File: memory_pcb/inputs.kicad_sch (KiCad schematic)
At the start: 12 parts, among them SW1 SW_Push, SW2 SW_Push, SW3 RotaryEncoder_Switch, U3 100SP3T2B4M6RE

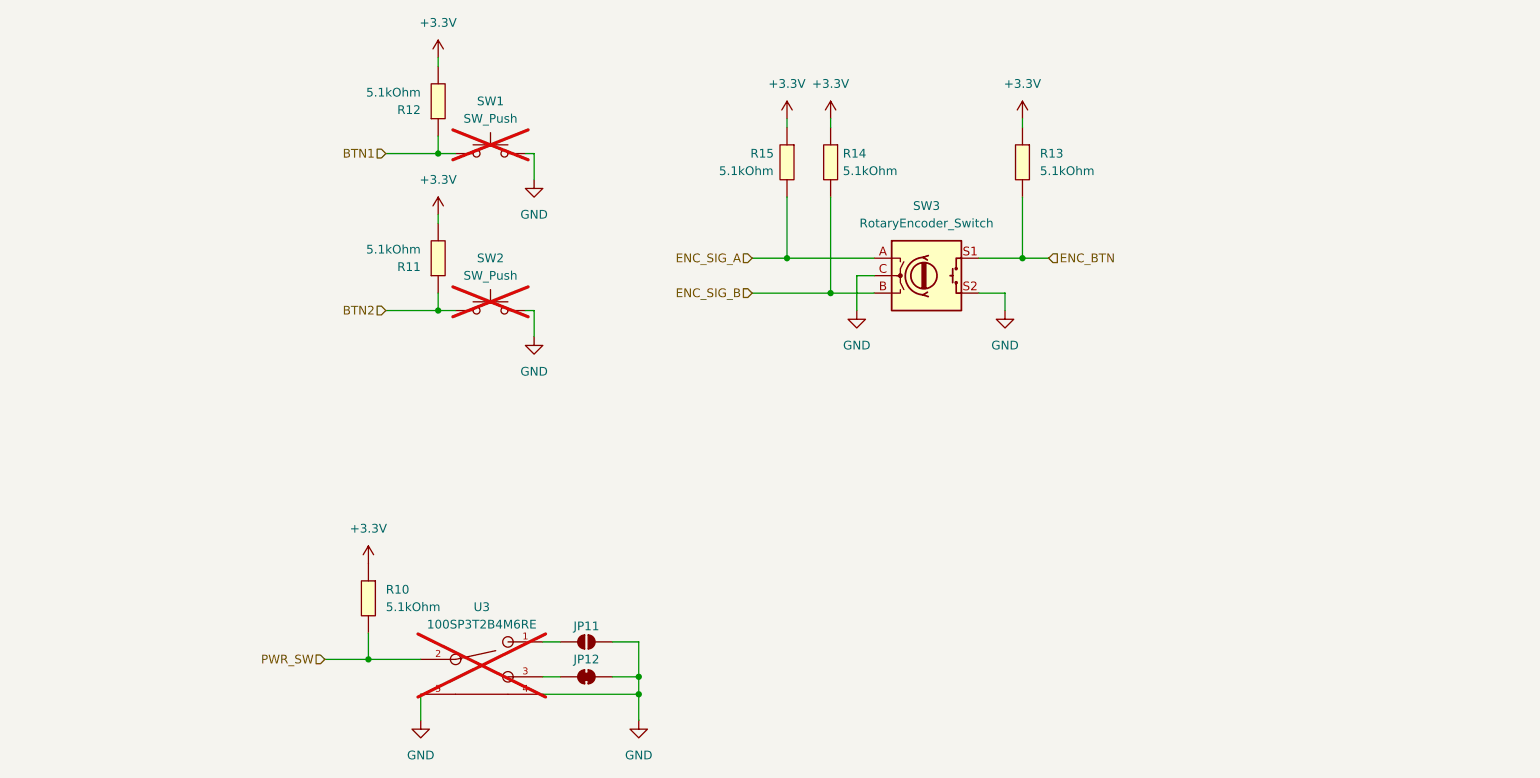
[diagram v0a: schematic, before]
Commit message: and so it begins
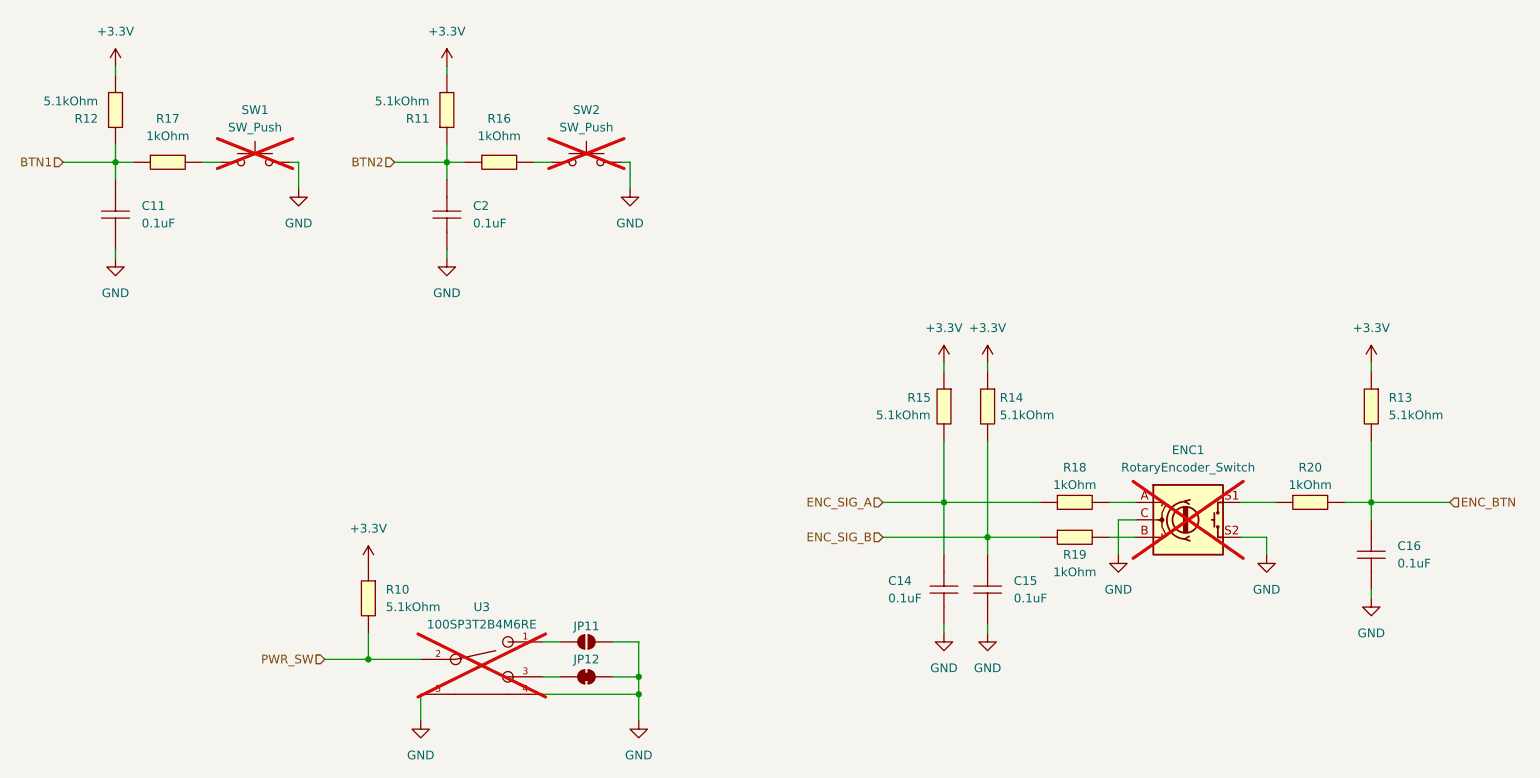
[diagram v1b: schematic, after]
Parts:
- added C11, C14, C15, C16, C2: 0.1uF, new_lib_footprint:C0402, symbol new_lib_symbol:CL05B104KO5NNNC
- added R16, R17, R18, R19, R20: 1kOhm, new_lib_footprint:R0603, symbol new_lib_symbol:0603WAF1001T5E
- ENC1: renamed from SW3; footprint (none) -> Rotary_Encoder:RotaryEncoder_Alps_EC11E-Switch_Vertical_H20mm; now not fitted
- U3: footprint new_lib_footprint:SW-TH_100SP3T2B4M6RE -> new_lib_footprint:MTS-102-C3
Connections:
- net BTN1: now also C11.2, R17.1; no longer SW1.1
- net BTN2: now also C2.2, R16.1; no longer SW2.1
- net ENC_BTN: now also C16.2, R20.2; no longer ENC1.S1
- net ENC_SIG_A: now also C14.2, R18.1; no longer ENC1.A
- net ENC_SIG_B: now also C15.2, R19.1; no longer ENC1.B
- net GND: now also C11.1, C14.1, C15.1, C16.1, C2.1
- new net: ENC1.B, R19.2
- new net: ENC1.S1, R20.1
- new net: R17.2, SW1.1
- new net: ENC1.A, R18.2
- new net: R16.2, SW2.1
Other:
- moved on the sheet: R11, R12, R13, R14, R15, SW1, SW2
